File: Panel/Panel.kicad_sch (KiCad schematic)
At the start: 130 parts, among them J1 Conn_01x02_Male, J2 Conn_01x02_Female, J3 Conn_01x10_Male, J4 Conn_01x04_Male, J5 Conn_01x04_Male, Q1 MTP4835I3, Q10 SSM3J332R, Q11 S8050, Q12 SSM3J332R, Q13 S8050, Q14 S8050, Q15 BSS138, Q2 BSS138, Q3 MTP4835I3, Q4 SSM3J332R, Q5 2SC3265, Q6 S8050, Q7 SSM3J332R, Q8 MTP4835I3, Q9 S8050, SW1 SW_DIP_x05, SW2 SW_SPDT, SW3 SW_SPDT_White, SW4 SW_SPST, U1 MC34063AD, U2 AZ1084CD-3.3, U3 STM32G050F6P6, U4 MAX3485, U5 NJU6319AE, Y1 16MHz

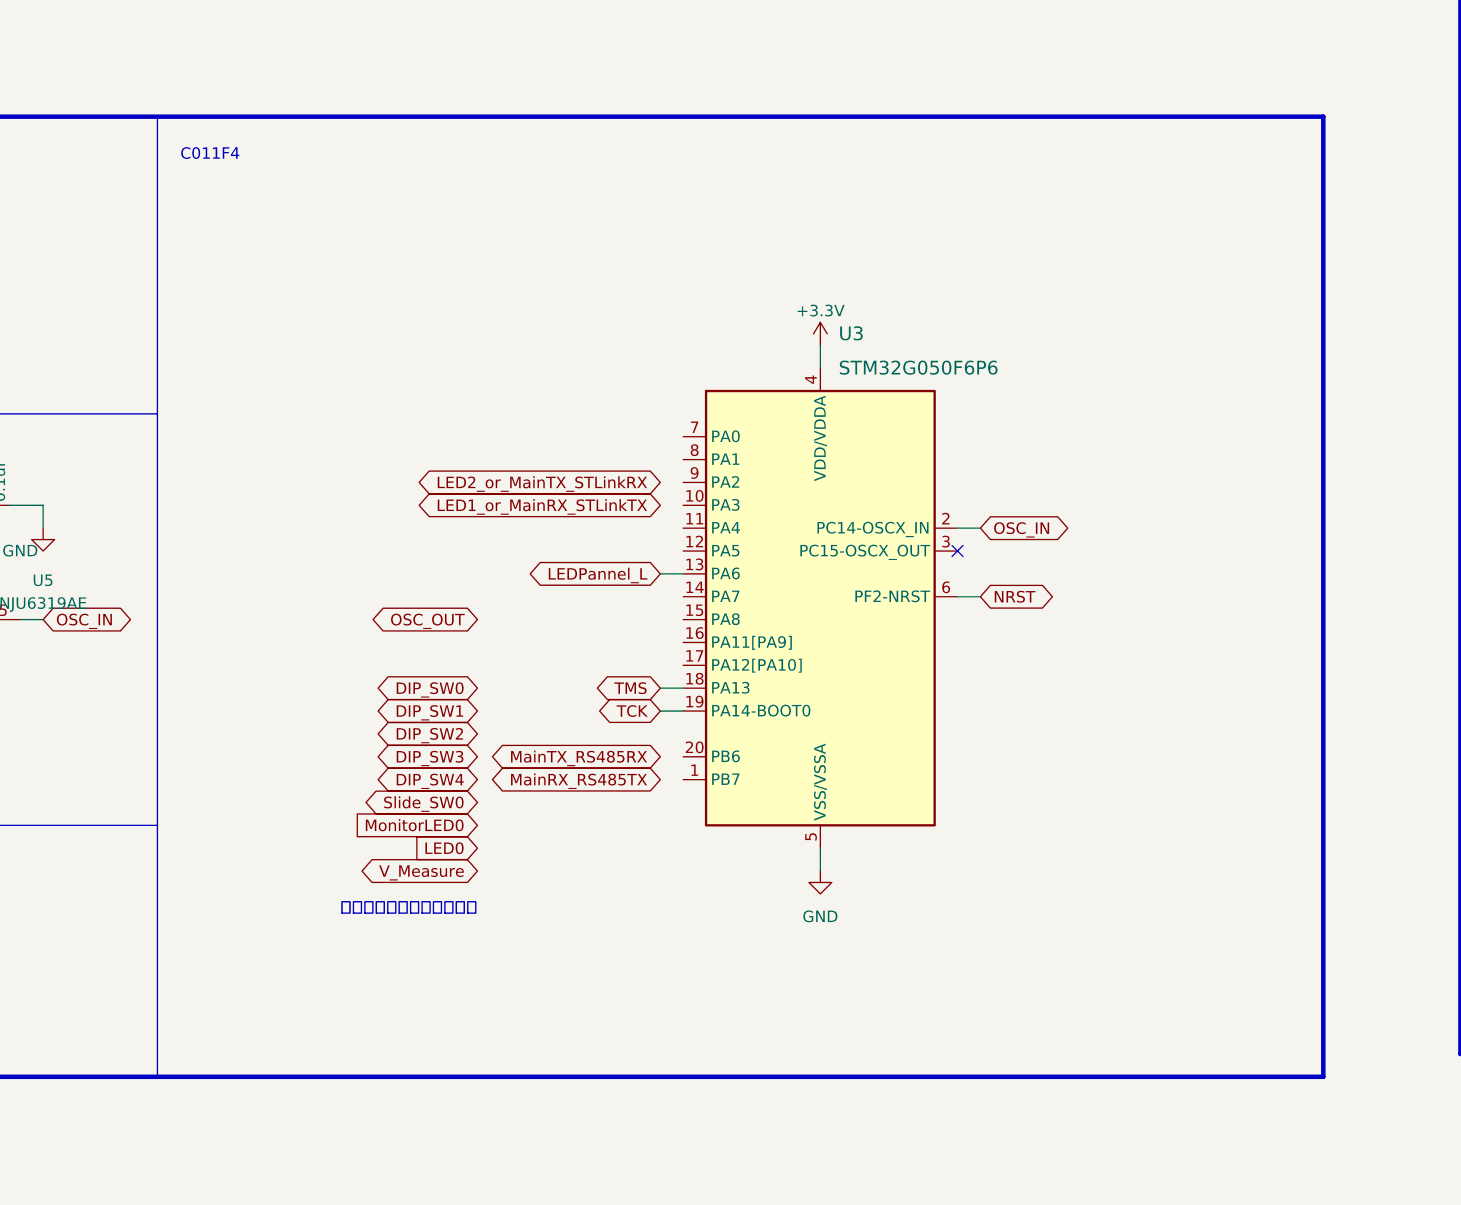
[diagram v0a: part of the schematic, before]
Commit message: LargeMD
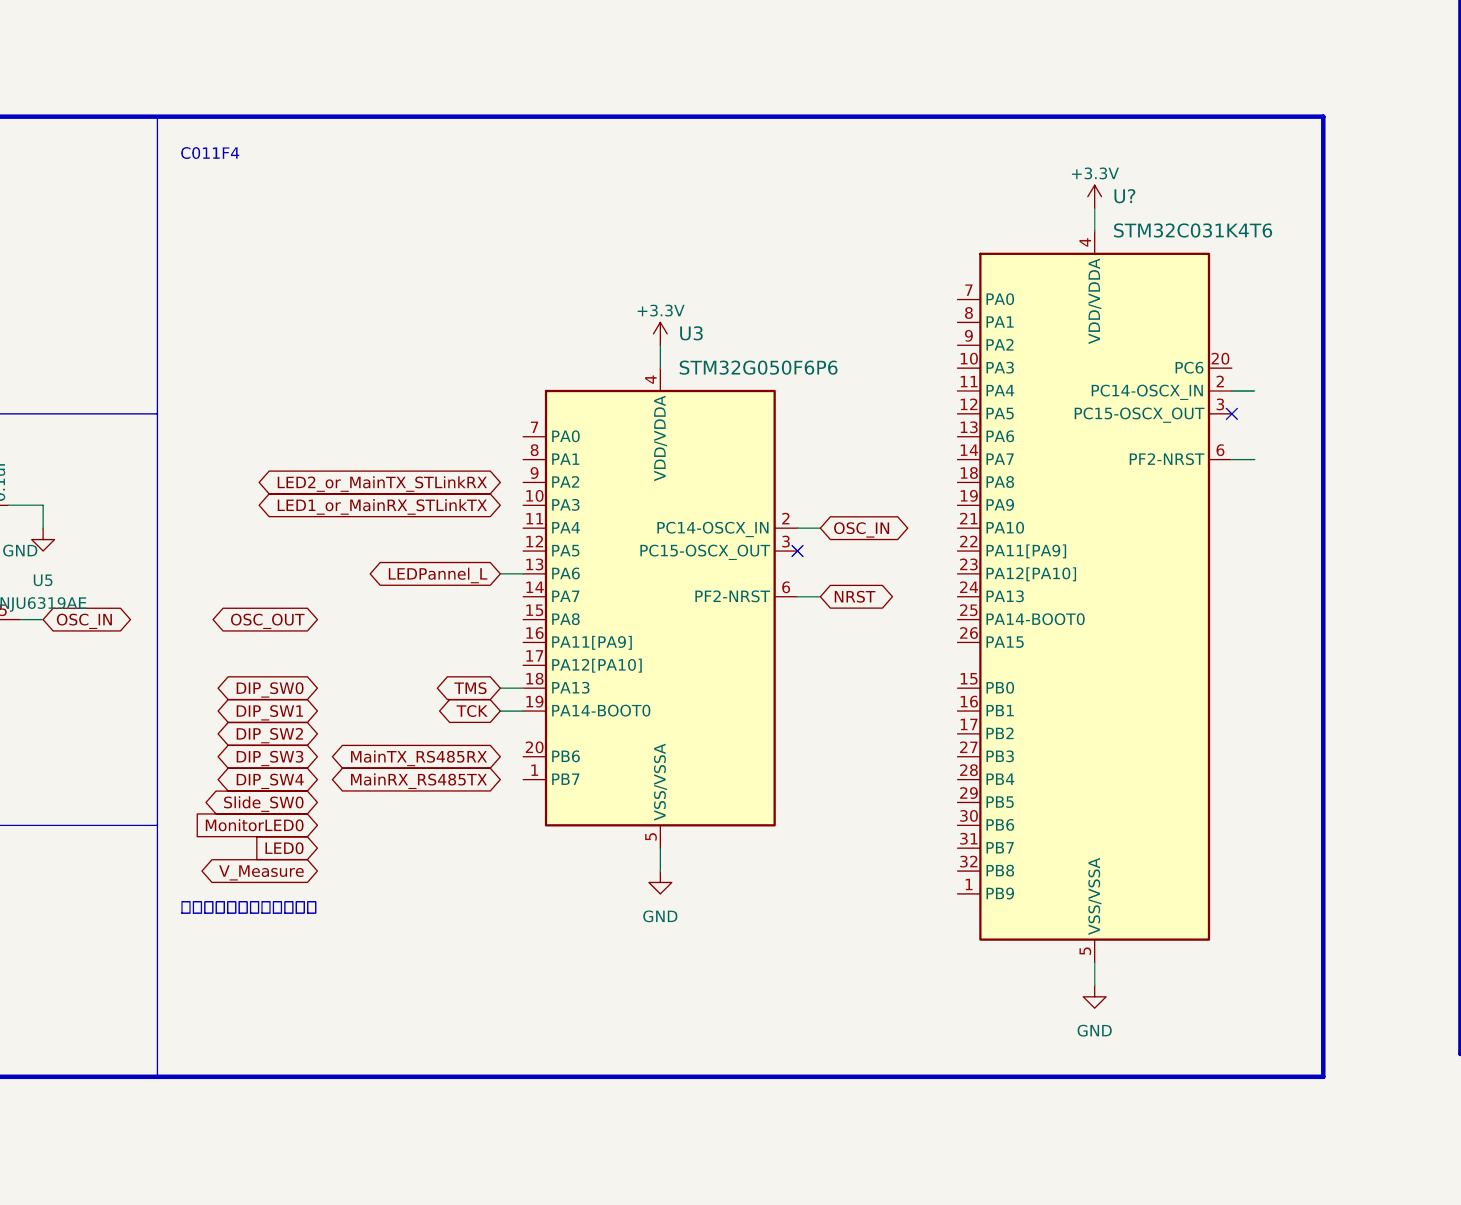
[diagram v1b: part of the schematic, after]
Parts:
- added U?: STM32C031K4T6, Package_QFP:LQFP-32_7x7mm_P0.8mm, symbol STM32C031K4T6:STM32C031K4T6
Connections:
- net +3.3V: now also U?.4 (VDD/VDDA)
- net GND: now also U?.5 (VSS/VSSA)
- no-connect marks 6 -> 7
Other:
- moved on the sheet: U3
